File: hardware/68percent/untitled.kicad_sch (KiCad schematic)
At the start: 2 parts

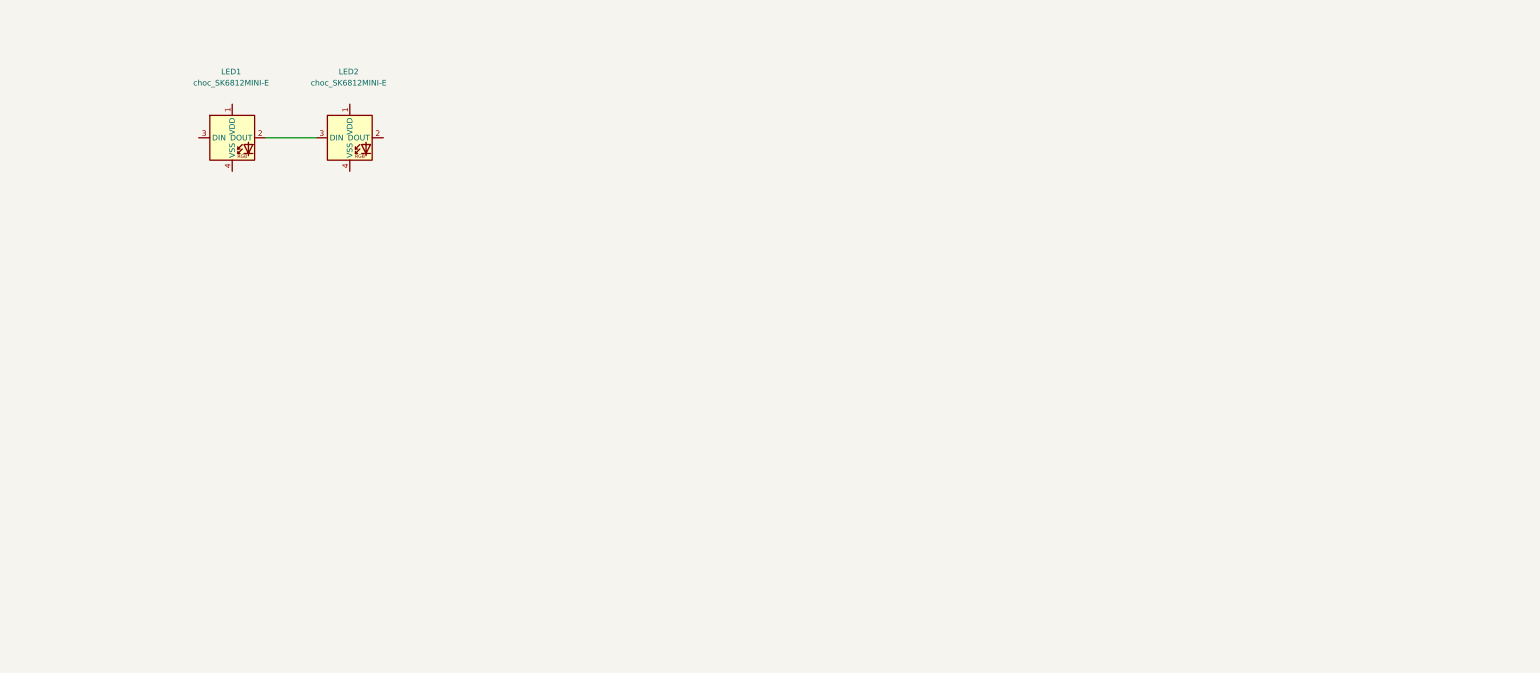
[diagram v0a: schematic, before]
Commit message: LEDs
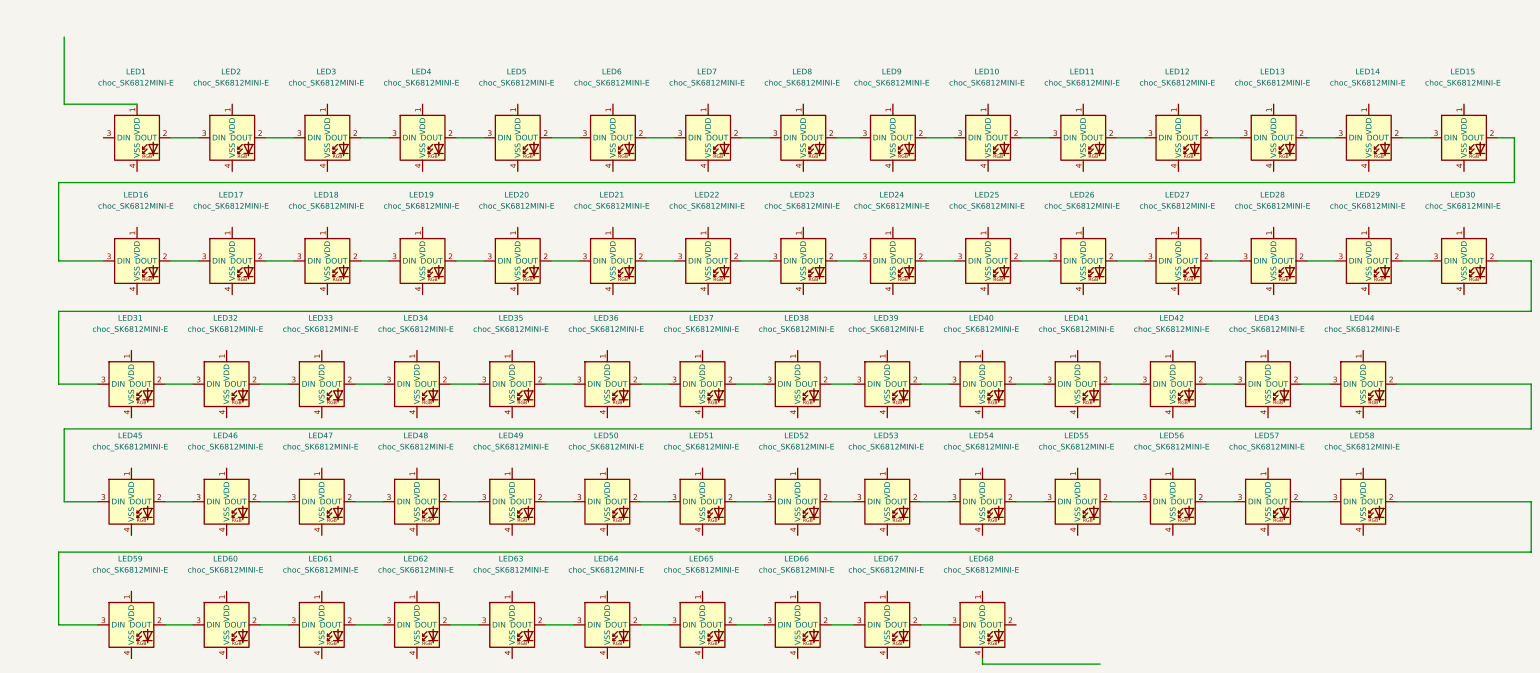
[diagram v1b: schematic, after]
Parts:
- added LED10, LED11, LED12, LED13, LED14, LED15, LED16, LED17, LED18, LED19, LED20, LED21, LED22, LED23, LED24, LED25, LED26, LED27, LED28, LED29, LED3, LED30, LED31, LED32, LED33, LED34, LED35, LED36, LED37, LED38, LED39, LED4, LED40, LED41, LED42, LED43, LED44, LED45, LED46, LED47, LED48, LED49, LED5, LED50, LED51, LED52, LED53, LED54, LED55, LED56, LED57, LED58, LED59, LED6, LED60, LED61, LED62, LED63, LED64, LED65, LED66, LED67, LED68, LED7, LED8, LED9: choc_SK6812MINI-E, PCM_marbastlib-choc:LED_choc_6028R, symbol PCM_marbastlib-choc:choc_SK6812MINI-E
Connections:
- net at LED2.2 (DOUT): now also LED3.3 (DIN)
- new net: LED42.2 (DOUT), LED43.3 (DIN)
- new net: LED41.2 (DOUT), LED42.3 (DIN)
- new net: LED16.2 (DOUT), LED17.3 (DIN)
- new net: LED15.2 (DOUT), LED16.3 (DIN)
- new net: LED19.2 (DOUT), LED20.3 (DIN)
- new net: LED18.2 (DOUT), LED19.3 (DIN)
- new net: LED40.2 (DOUT), LED41.3 (DIN)
- new net: LED67.2 (DOUT), LED68.3 (DIN)
- new net: LED55.2 (DOUT), LED56.3 (DIN)
- new net: LED54.2 (DOUT), LED55.3 (DIN)
- new net: LED11.2 (DOUT), LED12.3 (DIN)
- new net: LED10.2 (DOUT), LED11.3 (DIN)
- new net: LED25.2 (DOUT), LED26.3 (DIN)
- new net: LED24.2 (DOUT), LED25.3 (DIN)
- new net: LED47.2 (DOUT), LED48.3 (DIN)
- new net: LED46.2 (DOUT), LED47.3 (DIN)
- new net: LED27.2 (DOUT), LED28.3 (DIN)
- new net: LED26.2 (DOUT), LED27.3 (DIN)
- new net: LED57.2 (DOUT), LED58.3 (DIN)
- new net: LED56.2 (DOUT), LED57.3 (DIN)
- new net: LED13.2 (DOUT), LED14.3 (DIN)
- new net: LED12.2 (DOUT), LED13.3 (DIN)
- new net: LED14.2 (DOUT), LED15.3 (DIN)
- new net: LED29.2 (DOUT), LED30.3 (DIN)
- new net: LED28.2 (DOUT), LED29.3 (DIN)
- new net: LED53.2 (DOUT), LED54.3 (DIN)
- new net: LED7.2 (DOUT), LED8.3 (DIN)
- new net: LED6.2 (DOUT), LED7.3 (DIN)
- new net: LED34.2 (DOUT), LED35.3 (DIN)
- new net: LED33.2 (DOUT), LED34.3 (DIN)
- new net: LED4.2 (DOUT), LED5.3 (DIN)
- new net: LED3.2 (DOUT), LED4.3 (DIN)
- new net: LED36.2 (DOUT), LED37.3 (DIN)
- new net: LED35.2 (DOUT), LED36.3 (DIN)
- new net: LED61.2 (DOUT), LED62.3 (DIN)
- new net: LED60.2 (DOUT), LED61.3 (DIN)
- new net: LED38.2 (DOUT), LED39.3 (DIN)
- new net: LED37.2 (DOUT), LED38.3 (DIN)
- new net: LED10.3 (DIN), LED9.2 (DOUT)
- new net: LED21.2 (DOUT), LED22.3 (DIN)
- new net: LED20.2 (DOUT), LED21.3 (DIN)
- new net: LED62.2 (DOUT), LED63.3 (DIN)
- new net: LED64.2 (DOUT), LED65.3 (DIN)
- new net: LED63.2 (DOUT), LED64.3 (DIN)
- new net: LED8.2 (DOUT), LED9.3 (DIN)
- new net: LED59.2 (DOUT), LED60.3 (DIN)
- new net: LED58.2 (DOUT), LED59.3 (DIN)
- new net: LED23.2 (DOUT), LED24.3 (DIN)
- new net: LED66.2 (DOUT), LED67.3 (DIN)
- new net: LED30.2 (DOUT), LED31.3 (DIN)
- new net: LED32.2 (DOUT), LED33.3 (DIN)
- new net: LED31.2 (DOUT), LED32.3 (DIN)
- new net: LED45.2 (DOUT), LED46.3 (DIN)
- new net: LED44.2 (DOUT), LED45.3 (DIN)
- new net: LED50.2 (DOUT), LED51.3 (DIN)
- new net: LED49.2 (DOUT), LED50.3 (DIN)
- new net: LED65.2 (DOUT), LED66.3 (DIN)
- new net: LED52.2 (DOUT), LED53.3 (DIN)
- new net: LED22.2 (DOUT), LED23.3 (DIN)
- new net: LED39.2 (DOUT), LED40.3 (DIN)
- new net: LED5.2 (DOUT), LED6.3 (DIN)
- new net: LED17.2 (DOUT), LED18.3 (DIN)
- new net: LED51.2 (DOUT), LED52.3 (DIN)
- new net: LED48.2 (DOUT), LED49.3 (DIN)
- new net: LED43.2 (DOUT), LED44.3 (DIN)
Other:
- moved on the sheet: LED1, LED2

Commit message: traces
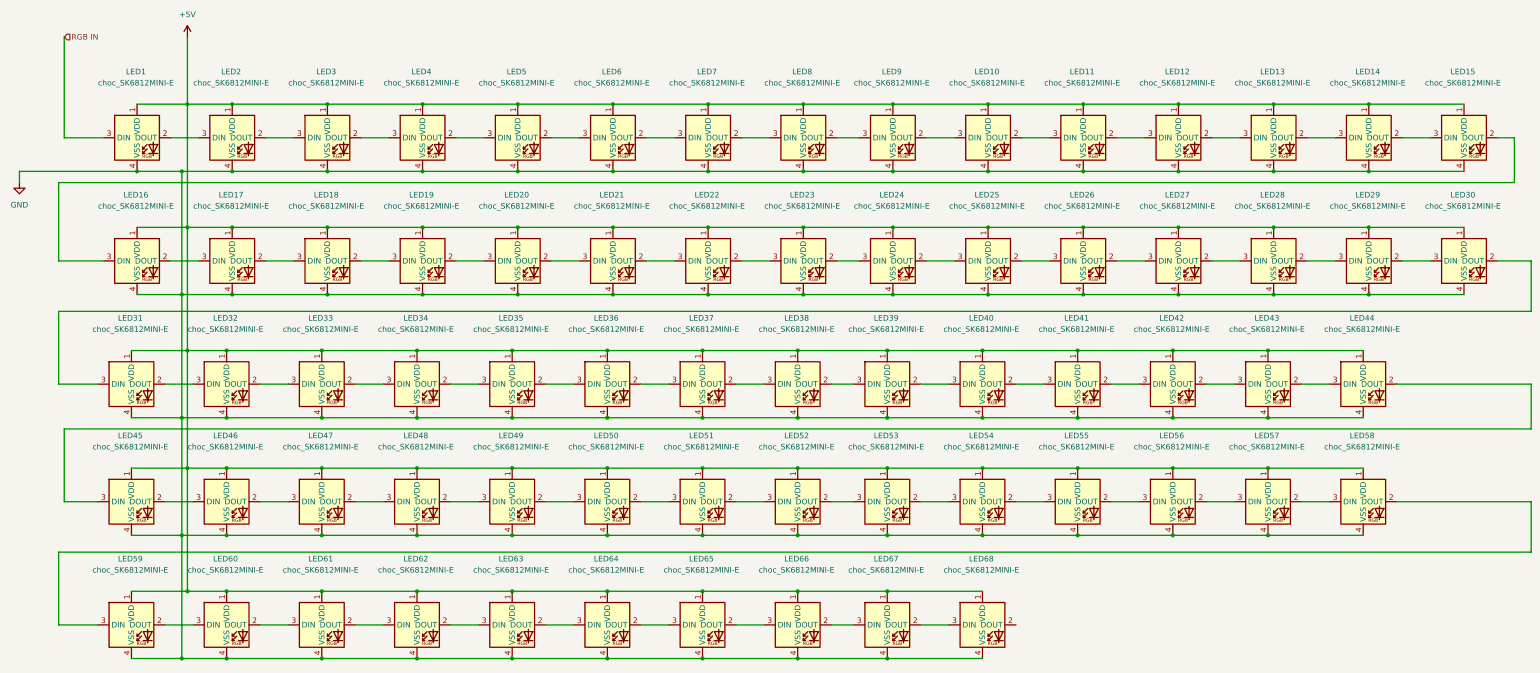
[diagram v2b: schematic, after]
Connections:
- net +5V: now reaches LED42.1 (VDD)
- net +5V: now also LED1.1 (VDD), LED10.1 (VDD), LED11.1 (VDD), LED12.1 (VDD), LED13.1 (VDD), LED14.1 (VDD), LED15.1 (VDD), LED16.1 (VDD), LED17.1 (VDD), LED18.1 (VDD), LED19.1 (VDD), LED2.1 (VDD), LED20.1 (VDD), LED21.1 (VDD), LED22.1 (VDD), LED23.1 (VDD), LED24.1 (VDD), LED25.1 (VDD), LED26.1 (VDD), LED27.1 (VDD), LED28.1 (VDD), LED29.1 (VDD), LED3.1 (VDD), LED30.1 (VDD), LED31.1 (VDD), LED32.1 (VDD), LED33.1 (VDD), LED34.1 (VDD), LED35.1 (VDD), LED36.1 (VDD), LED37.1 (VDD), LED38.1 (VDD), LED39.1 (VDD), LED4.1 (VDD), LED40.1 (VDD), LED41.1 (VDD), LED43.1 (VDD), LED44.1 (VDD), LED45.1 (VDD), LED46.1 (VDD), LED47.1 (VDD), LED48.1 (VDD), LED49.1 (VDD), LED5.1 (VDD), LED50.1 (VDD), LED51.1 (VDD), LED52.1 (VDD), LED53.1 (VDD), LED54.1 (VDD), LED55.1 (VDD), LED56.1 (VDD), LED57.1 (VDD), LED58.1 (VDD), LED59.1 (VDD), LED6.1 (VDD), LED60.1 (VDD), LED61.1 (VDD), LED62.1 (VDD), LED63.1 (VDD), LED64.1 (VDD), LED65.1 (VDD), LED66.1 (VDD), LED67.1 (VDD), LED68.1 (VDD), LED7.1 (VDD), LED8.1 (VDD), LED9.1 (VDD)
- net GND: now reaches LED42.4 (VSS)
- net GND: now also LED1.4 (VSS), LED10.4 (VSS), LED11.4 (VSS), LED12.4 (VSS), LED13.4 (VSS), LED14.4 (VSS), LED15.4 (VSS), LED16.4 (VSS), LED17.4 (VSS), LED18.4 (VSS), LED19.4 (VSS), LED2.4 (VSS), LED20.4 (VSS), LED21.4 (VSS), LED22.4 (VSS), LED23.4 (VSS), LED24.4 (VSS), LED25.4 (VSS), LED26.4 (VSS), LED27.4 (VSS), LED28.4 (VSS), LED29.4 (VSS), LED3.4 (VSS), LED30.4 (VSS), LED31.4 (VSS), LED32.4 (VSS), LED33.4 (VSS), LED34.4 (VSS), LED35.4 (VSS), LED36.4 (VSS), LED37.4 (VSS), LED38.4 (VSS), LED39.4 (VSS), LED4.4 (VSS), LED40.4 (VSS), LED41.4 (VSS), LED43.4 (VSS), LED44.4 (VSS), LED45.4 (VSS), LED46.4 (VSS), LED47.4 (VSS), LED48.4 (VSS), LED49.4 (VSS), LED5.4 (VSS), LED50.4 (VSS), LED51.4 (VSS), LED52.4 (VSS), LED53.4 (VSS), LED54.4 (VSS), LED55.4 (VSS), LED56.4 (VSS), LED57.4 (VSS), LED58.4 (VSS), LED59.4 (VSS), LED6.4 (VSS), LED60.4 (VSS), LED61.4 (VSS), LED62.4 (VSS), LED63.4 (VSS), LED64.4 (VSS), LED65.4 (VSS), LED66.4 (VSS), LED67.4 (VSS), LED68.4 (VSS), LED7.4 (VSS), LED8.4 (VSS), LED9.4 (VSS)
- net RGB IN: now reaches LED1.3 (DIN)
